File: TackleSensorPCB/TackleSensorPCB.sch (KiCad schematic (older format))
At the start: 26 parts, among them J1 PJ-037A, J2 Conn_01x03_Male, J3 Conn_01x04_Male, J4 Conn_01x07_Male, Q1 2N7002, Q2 2N7002, SW1 SW_DPST_x2, U1 TPS62172DSG, U2 MSP430FR2433IRGER, U3 MMA8452QR1

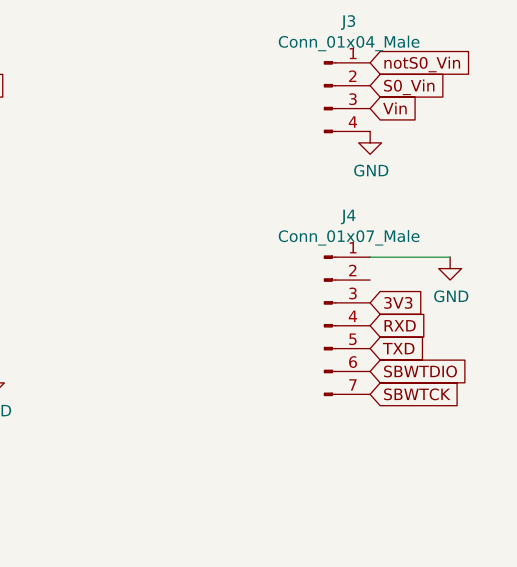
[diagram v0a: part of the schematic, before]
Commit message: Created First Revision of PCB
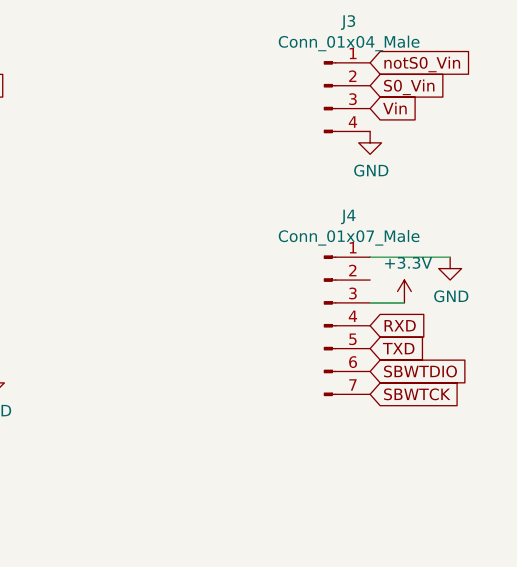
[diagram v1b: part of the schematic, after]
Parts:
- J4: footprint Connector_PinHeader_2.54mm:PinHeader_1x07_P2.54mm_Horizontal -> Connector_PinHeader_2.54mm:PinHeader_1x07_P2.54mm_Vertical
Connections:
- net 3V3 is gone; now on net +3V3: J4.3 (Pin_3)
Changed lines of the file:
@@
 F 0 "J4" H 9908 6331 50  0000 C CNN
 F 1 "Conn_01x07_Male" H 9908 6240 50  0000 C CNN
-F 2 "Connector_PinHeader_2.54mm:PinHeader_1x07_P2.54mm_Horizontal" H 9800 5850 50  0001 C CNN
+F 2 "Connector_PinHeader_2.54mm:PinHeader_1x07_P2.54mm_Vertical" H 9800 5850 50  0001 C CNN
 F 3 "~" H 9800 5850 50  0001 C CNN
 	1    9800 5850
@@
 	1    0    0    -1
 $EndComp
-Text GLabel 10000 5750 2    50   Input ~ 0
-3V3
 Text GLabel 10000 5850 2    50   Input ~ 0
 RXD
@@
 	1400 1650 1650 1650
 Connection ~ 1650 1650
+$Comp
+L power:+3.3V #PWR?
+U 1 1 5F87745C
+P 10150 5750
+F 0 "#PWR?" H 10150 5600 50  0001 C CNN
+F 1 "+3.3V" H 10165 5923 50  0000 C CNN
+F 2 "" H 10150 5750 50  0001 C CNN
+F 3 "" H 10150 5750 50  0001 C CNN
+	1    10150 5750
+	1    0    0    -1
+$EndComp
+Wire Wire Line
+	10000 5750 10150 5750
 $EndSCHEMATC
